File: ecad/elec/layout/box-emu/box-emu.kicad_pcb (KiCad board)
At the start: 2 copper layers, 72.5 x 63.9 mm, 73 parts

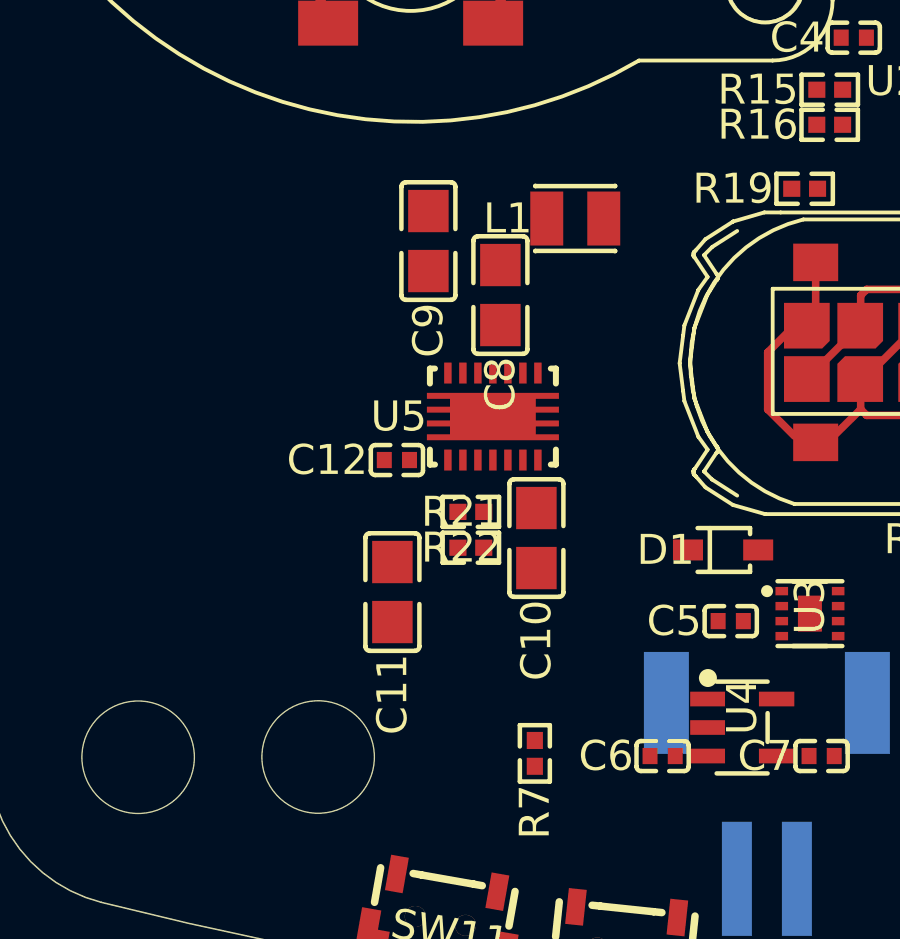
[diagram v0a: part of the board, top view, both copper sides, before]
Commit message: further layout changes
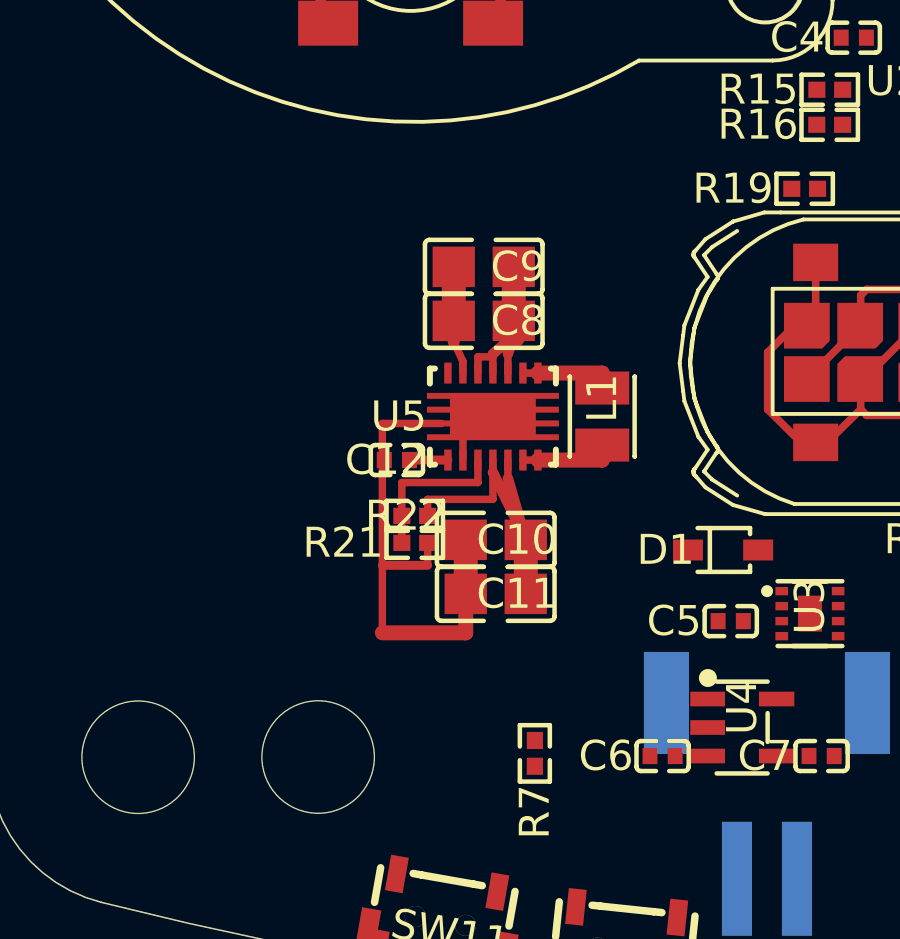
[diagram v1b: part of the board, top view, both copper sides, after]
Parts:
- moved L1 6.66 mm to (152.2, 123.9), turned to 270 degrees
- moved C11 3.45 mm to (148.7, 129.8), turned to 180 degrees
- moved R22 2.15 mm to (146.0, 127.2)
- moved R21 2.14 mm to (146.0, 128.1), turned to 0 degrees
- moved C9 2.04 mm to (148.3, 118.9), turned to 180 degrees
- moved C10 1.36 mm to (148.7, 128.0), turned to 180 degrees
- moved C8 1.02 mm to (148.3, 120.7), turned to 180 degrees
- turned C12 to 180 degrees
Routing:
- net gnd: track 0.00 -> 21.5 mm
- net vcc_5v: track 0.00 -> 11.1 mm
- net vbat: track 0.00 -> 7.45 mm
- net FB: track 0.00 -> 5.29 mm
- net 2: track 0.00 -> 3.15 mm
- net 1: track 0.00 -> 3.15 mm
